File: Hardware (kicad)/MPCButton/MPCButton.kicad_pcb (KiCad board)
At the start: 2 copper layers, 30 x 30 mm, 5 parts, among them P1 62100421921

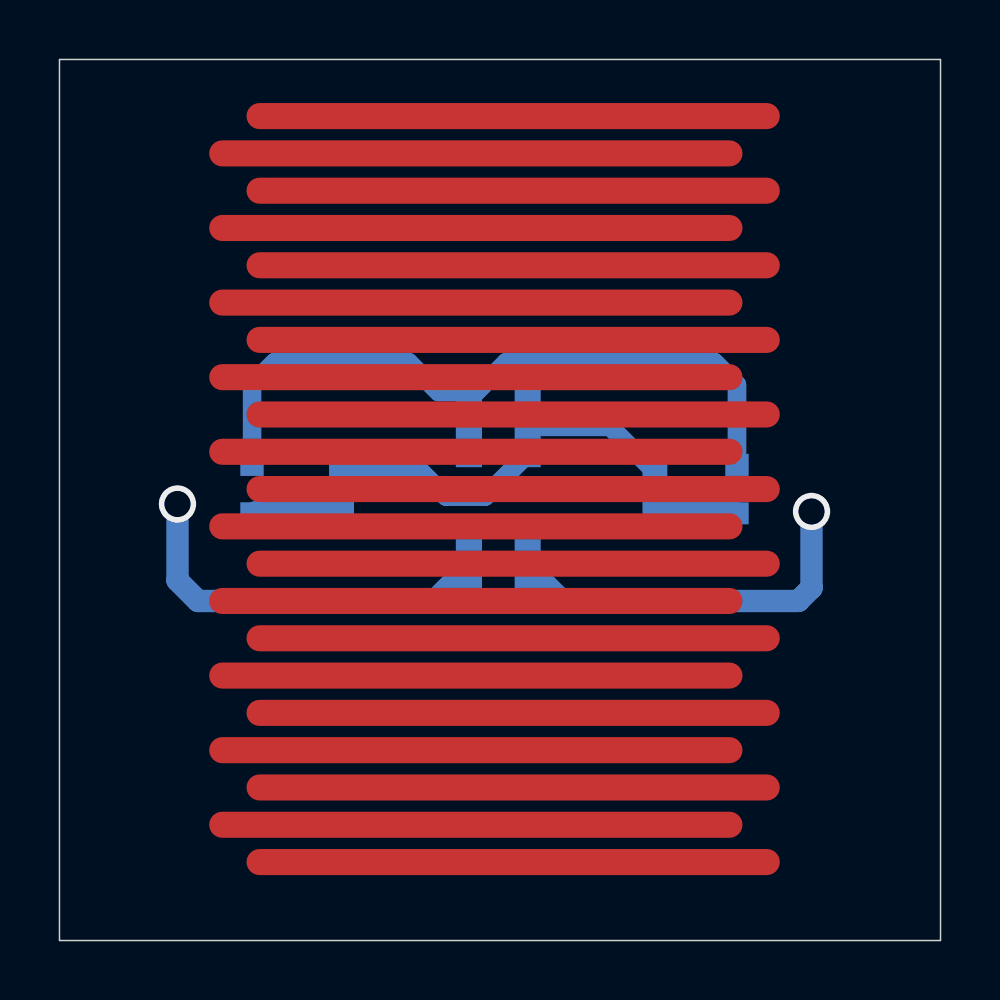
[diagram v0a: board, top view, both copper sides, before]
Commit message: fix kicad projects
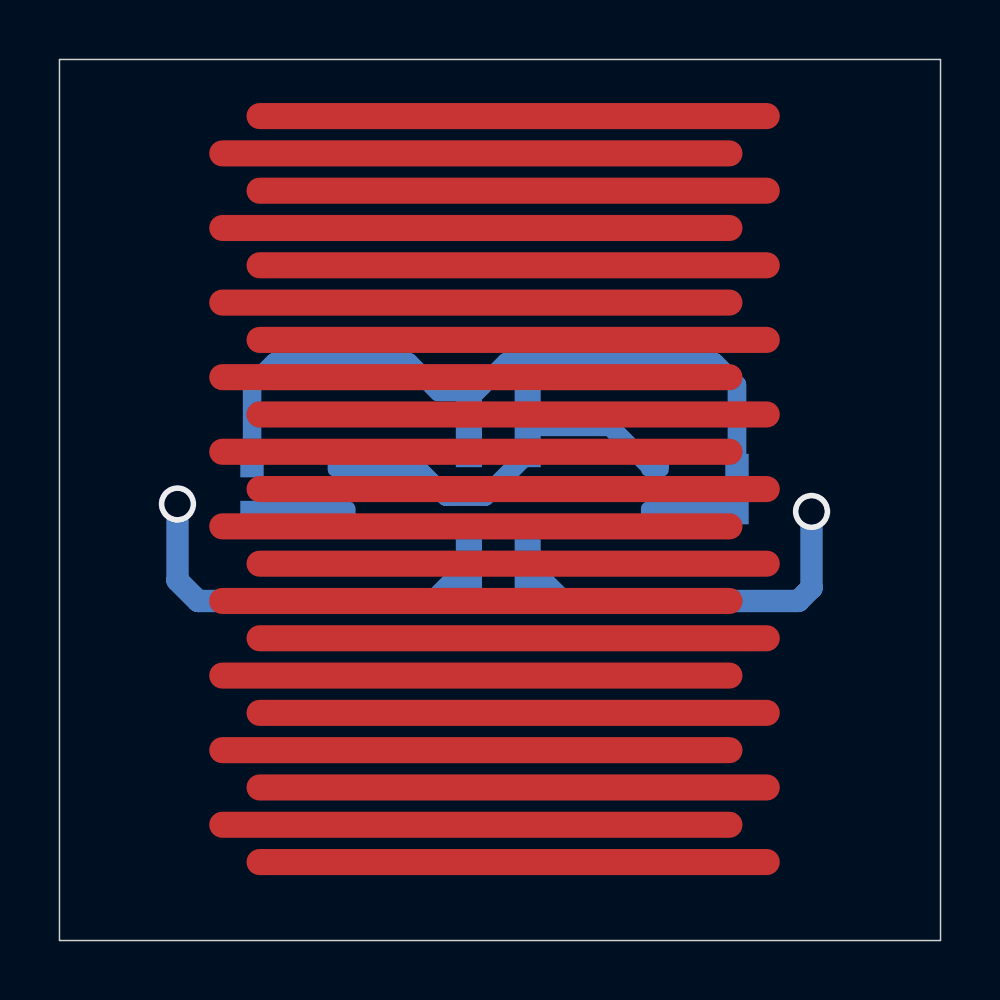
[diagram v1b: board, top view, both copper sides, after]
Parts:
- D1, D2: footprint Altium_WL-SMCC (rev24a):WL-SMCC_0603_150060xx73220 -> Wurth_WL-SMCW (rev24b):WL-SMCW_0603_150060xx75000
- R1, R2: footprint Passive SMD:RESC0603(1608)_N -> Resistor_SMD:R_0603_1608Metric_Pad0.98x0.95mm_HandSolder
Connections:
- net Btn_Output renamed /Btn_Output
- net Btn_Power renamed /Btn_Power
- net LED_GND renamed /LED_GND
- net LED_ON renamed /LED_ON
- net NetD1_2 renamed Net-(D1-A)
- net NetD2_2 renamed Net-(D2-A)
